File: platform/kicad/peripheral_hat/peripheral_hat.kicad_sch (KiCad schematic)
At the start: 25 parts, among them J1 CRJ032-1-TH, J2 Pi Header, T1 PT61018PEL, U2 ENC28J60x-SS

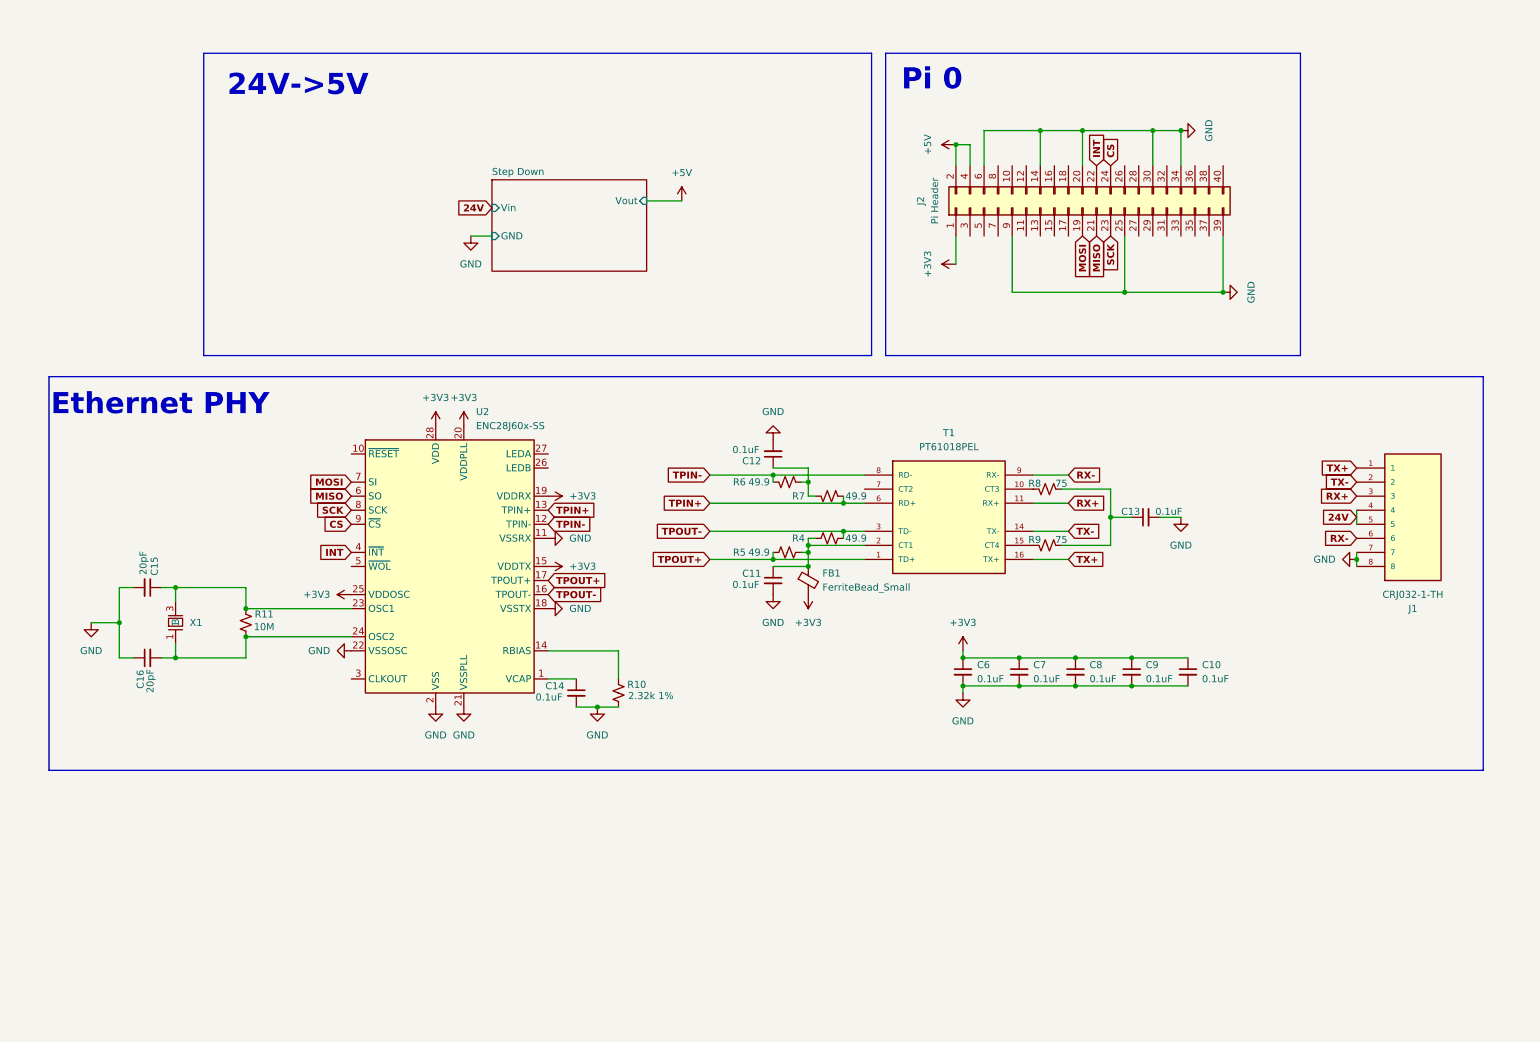
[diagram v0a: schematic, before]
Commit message: WIP
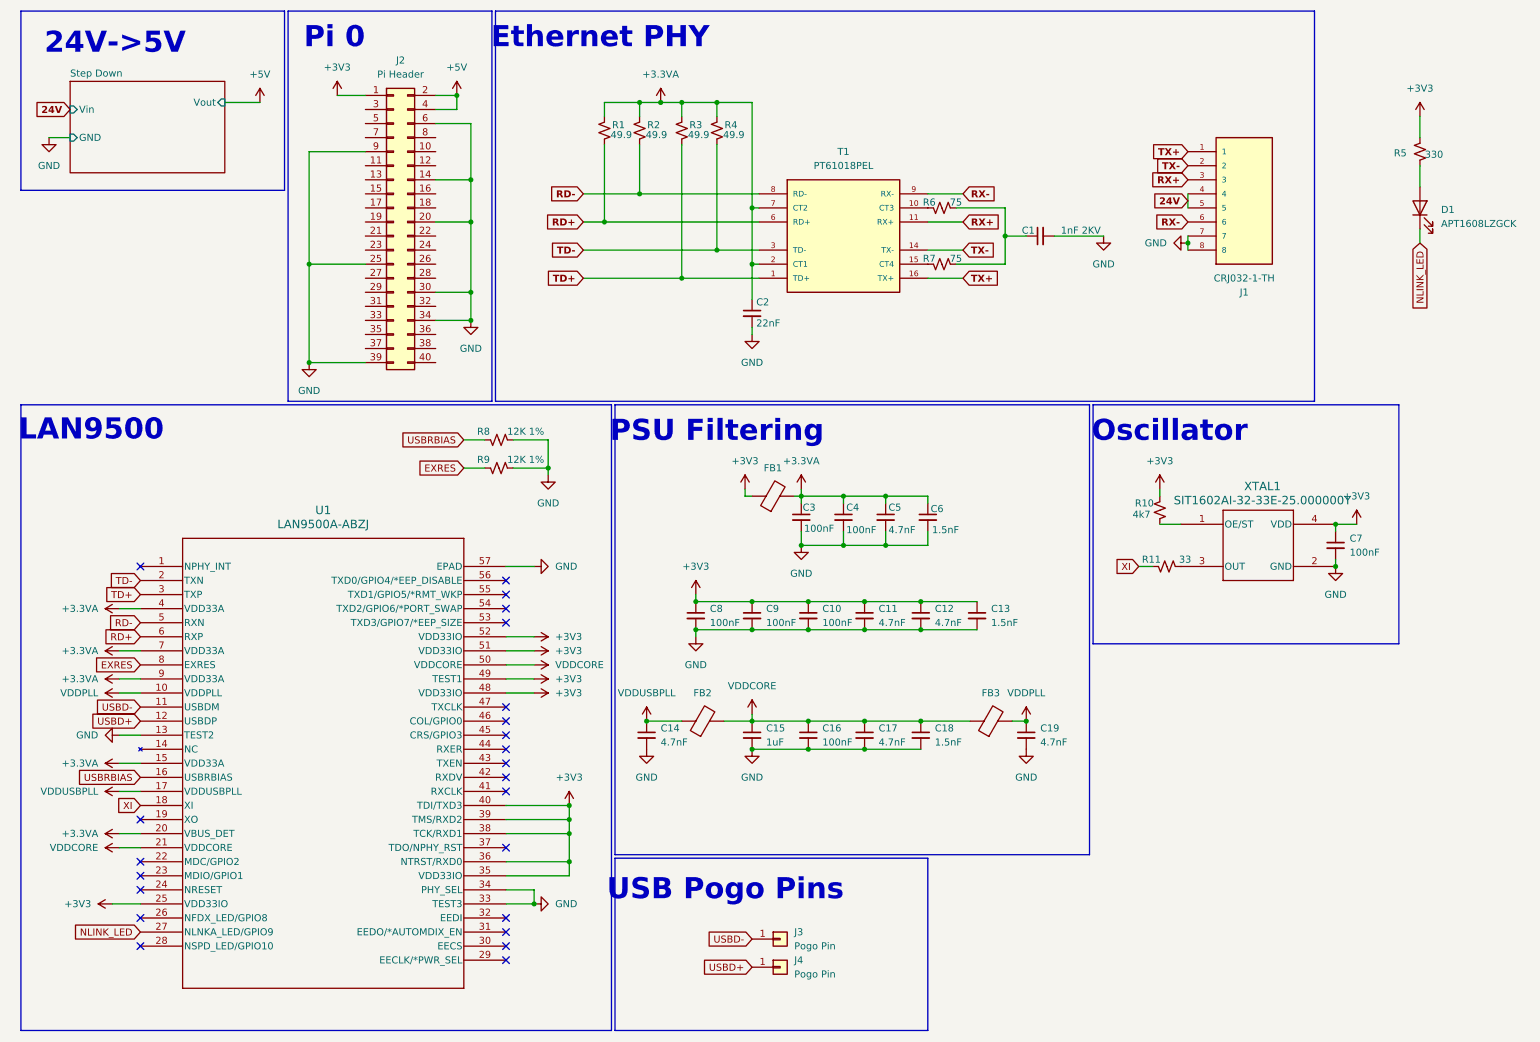
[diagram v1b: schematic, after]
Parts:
- removed C10: 0.1uF, Capacitor_SMD:C_0201_0603Metric, symbol Device:C_Small
- removed FB1: FerriteBead_Small, Resistor_SMD:R_0603_1608Metric, symbol Device:FerriteBead_Small
- removed R6, R7: 49.9, Resistor_SMD:R_0201_0603Metric, symbol Device:R_Small_US
- removed U2: ENC28J60x-SS, Package_SO:SSOP-28_5.3x10.2mm_P0.65mm, symbol Interface_Ethernet:ENC28J60x-SS
- removed X1: ~, AusOcean:X322525MOB4SI, symbol AusOcean:X322525MOB4SI
- added C13, C18, C6: 1.5nF, Capacitor_SMD:C_0402_1005Metric, symbol Device:C_Small
- added C17, C19, C5: 4.7nF, Capacitor_SMD:C_0402_1005Metric, symbol Device:C_Small
- added C3, C4, C7: 100nF, Capacitor_SMD:C_0402_1005Metric, symbol Device:C_Small
- added D1: APT1608LZGCK, Capacitor_SMD:C_0805_2012Metric, symbol Device:LED
- added FB1, FB2, FB3: MMZ1608B121CTAH0, Capacitor_SMD:C_0603_1608Metric, symbol Device:FerriteBead
- added J3, J4: Pogo Pin, AusOcean:YZ70115093P-02, symbol Connector_Generic:Conn_01x01
- added R1, R2, R3: 49.9, Resistor_SMD:R_0402_1005Metric, symbol Device:R_Small_US
- added R8, R9: 12K 1%, Resistor_SMD:R_0402_1005Metric, symbol Device:R_Small_US
- added U1: LAN9500A-ABZJ, AusOcean:QFN56_8X8MC_MCH, symbol AusOcean:LAN9500A-ABZJ
- added XTAL1: SIT1602AI-32-33E-25.000000Y, AusOcean:SON4_SIT1602-3_SIT, symbol AusOcean:SIT1602AI-32-33E-25.000000Y
- C1: renamed from C13; value 0.1uF -> 1nF 2KV; footprint Capacitor_SMD:C_0201_0603Metric -> Capacitor_SMD:C_0402_1005Metric
- C10: renamed from C8; value 0.1uF -> 100nF; footprint Capacitor_SMD:C_0201_0603Metric -> Capacitor_SMD:C_0402_1005Metric
- C11: renamed from C9; value 0.1uF -> 4.7nF; footprint Capacitor_SMD:C_0201_0603Metric -> Capacitor_SMD:C_0402_1005Metric
- C12, C14: value 0.1uF -> 4.7nF; footprint Capacitor_SMD:C_0201_0603Metric -> Capacitor_SMD:C_0402_1005Metric
- C15: value 20pF -> 1uF; footprint Capacitor_SMD:C_0201_0603Metric -> Capacitor_SMD:C_0402_1005Metric
- C16: value 20pF -> 100nF; footprint Capacitor_SMD:C_0201_0603Metric -> Capacitor_SMD:C_0402_1005Metric
- C2: renamed from C11; value 0.1uF -> 22nF; footprint Capacitor_SMD:C_0201_0603Metric -> Capacitor_SMD:C_0402_1005Metric
- C8: renamed from C6; value 0.1uF -> 100nF; footprint Capacitor_SMD:C_0201_0603Metric -> Capacitor_SMD:C_0402_1005Metric
- C9: renamed from C7; value 0.1uF -> 100nF; footprint Capacitor_SMD:C_0201_0603Metric -> Capacitor_SMD:C_0402_1005Metric
- R10: value 2.32k 1% -> 4k7; footprint Resistor_SMD:R_0201_0603Metric -> Resistor_SMD:R_0402_1005Metric
- R11: value 10M -> 33; footprint Resistor_SMD:R_0201_0603Metric -> Resistor_SMD:R_0402_1005Metric
- R4: footprint Resistor_SMD:R_0201_0603Metric -> Resistor_SMD:R_0402_1005Metric
- R5: value 49.9 -> 330; footprint Resistor_SMD:R_0201_0603Metric -> Resistor_SMD:R_0402_1005Metric
- R6: renamed from R8; footprint Resistor_SMD:R_0201_0603Metric -> Resistor_SMD:R_0402_1005Metric
- R7: renamed from R9; footprint Resistor_SMD:R_0201_0603Metric -> Resistor_SMD:R_0402_1005Metric
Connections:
- net +3V3: now also C12.1, R10.2, R5.2, C13.1, C7.1, FB1.1, U1.25 (VDD33IO), U1.35 (VDD33IO), U1.36 (NTRST/RXD0), U1.38 (TCK/RXD1), U1.39 (TMS/RXD2), U1.40 (TDI/TXD3), U1.48 (VDD33IO), U1.49 (TEST1), U1.51 (VDD33IO), U1.52 (VDD33IO), XTAL1.4 (VDD)
- net GND: now also C16.2, C13.2, C17.2, C18.2, C19.2, C3.2, C4.2, C5.2, C6.2, C7.2, R8.1, R9.1, U1.13 (TEST2), U1.33 (TEST3), U1.34 (PHY_SEL), U1.57 (EPAD), XTAL1.2 (GND); no longer C16.1, R10.1
- net at R11.1: now also XTAL1.3 (OUT); no longer C16.2
- net VDDCORE: now reaches C15.1
- net VDDCORE: now also C16.1, C17.1, C18.1, FB2.2, FB3.1, U1.21 (VDDCORE), U1.50 (VDDCORE); no longer R11.2
- net +3.3VA: now reaches C2.1, T1.2 (CT1)
- net +3.3VA: now also R4.2, T1.7 (CT2), C3.1, C4.1, C5.1, C6.1, FB1.2, R1.2, R2.2, R3.2, U1.15 (VDD33A), U1.20 (VBUS_DET), U1.4 (VDD33A), U1.7 (VDD33A), U1.9 (VDD33A); no longer R4.1, R5.2
- net VDDUSBPLL: now reaches C14.1
- net VDDUSBPLL: now also FB2.1, U1.17 (VDDUSBPLL)
- net CS: no longer names the net of J2.24 (Pin_24)
- net INT: no longer names the net of J2.22 (Pin_22)
- net MISO: no longer names the net of J2.21 (Pin_21)
- net MOSI: no longer names the net of J2.19 (Pin_19)
- net SCK: no longer names the net of J2.23 (Pin_23)
- net TPIN+ renamed RD+
- net RD+: now also R1.1, U1.6 (RXP)
- net TPIN- renamed RD-
- net RD-: now also R2.1, U1.5 (RXN)
- net TPOUT+: no longer names the net of R5.1
- net TPOUT+: now also D1.2 (A); no longer T1.1 (TD+)
- net TPOUT- renamed TD-
- net TD-: now also R4.1, U1.2 (TXN); no longer R4.2
- new net: R10.1, XTAL1.1 (OE/ST)
- new net EXRES: R9.2, U1.8 (EXRES)
- new net NLINK_LED: D1.1 (K), U1.27 (NLNKA_LED/GPIO9)
- new net TD+: R3.1, T1.1 (TD+), U1.3 (TXP)
- new net USBD+: J4.1 (Pin_1), U1.12 (USBDP)
- new net USBD-: J3.1 (Pin_1), U1.11 (USBDM)
- new net USBRBIAS: R8.2, U1.16 (USBRBIAS)
- new net VDDPLL: C19.1, FB3.2, U1.10 (VDDPLL)
- new net XI: R11.2, U1.18 (XI)
- no-connect marks 0 -> 23
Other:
- note added: "LAN9500"
- note added: "Oscillator"
- note added: "PSU Filtering"
- note added: "USB Pogo Pins"
- moved on the sheet: C1, C10, C11, C2, C8, C9, J1, J2, R6, R7, T1
